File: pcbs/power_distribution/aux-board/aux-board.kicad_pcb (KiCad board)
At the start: 2 copper layers, 85 x 56 mm, 16 parts, among them J1 Conn_01x02, J2 Raspberry Pi - Hat Template -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, J3 Conn_01x03, J4 Conn_01x03, J5 Conn_01x03, J6 Conn_01x03, J7 Conn_01x03, SW1 SW_Push, SW2 SW_Push, U1 YAAJ_WeAct_BlackPill_Part_Like

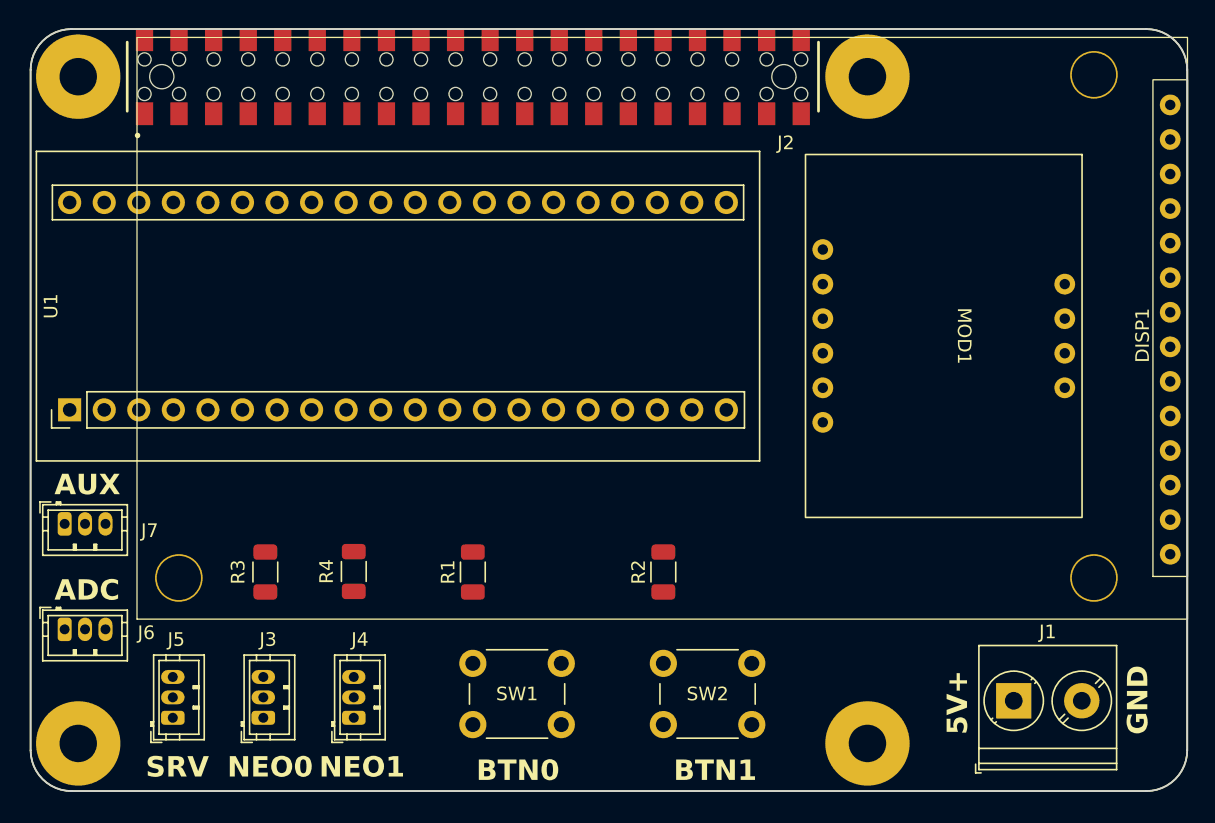
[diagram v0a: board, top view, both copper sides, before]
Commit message: PCB update.
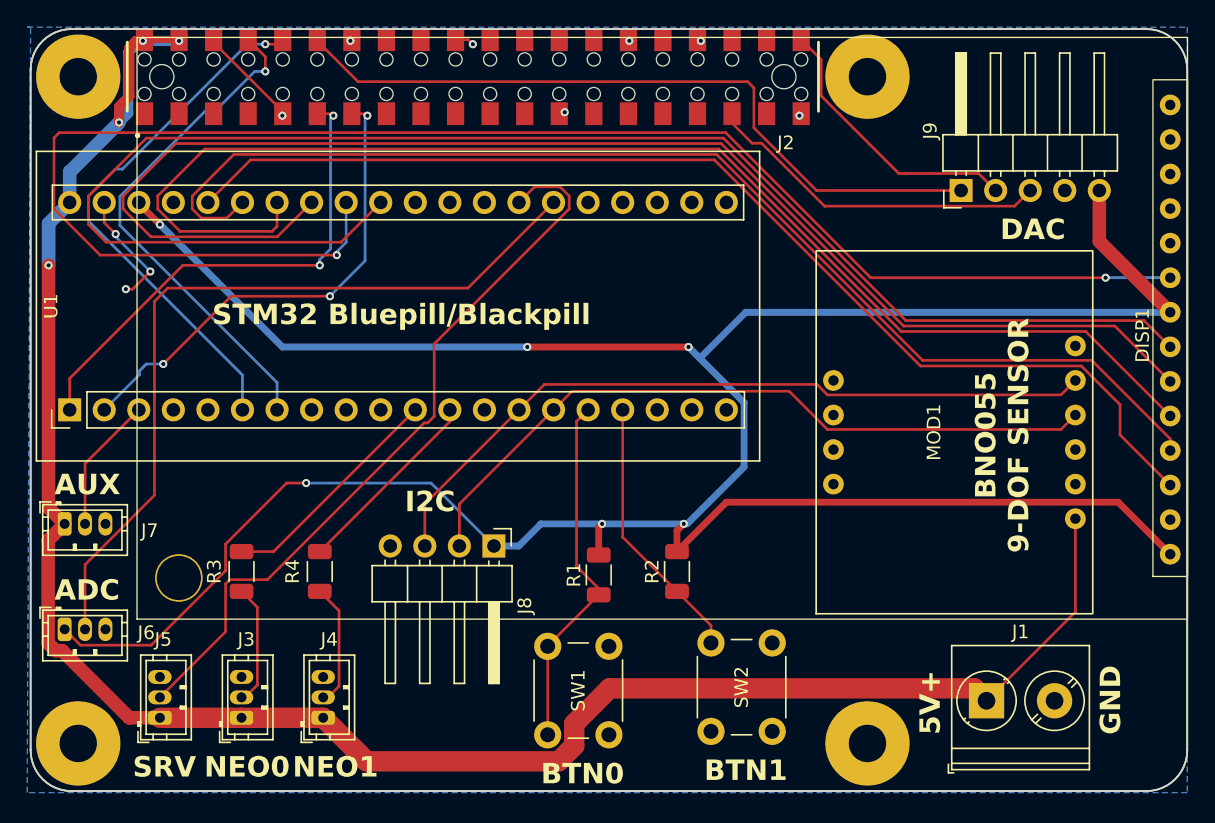
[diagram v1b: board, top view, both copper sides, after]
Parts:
- added J8: Conn_01x04, Connector_PinHeader_2.54mm:PinHeader_1x04_P2.54mm_Horizontal, F.Cu at (71.0, 76.6)
- added J9: Conn_01x05, Connector_PinHeader_2.54mm:PinHeader_1x05_P2.54mm_Horizontal, F.Cu at (105.4, 50.5)
- moved MOD1 27.1 mm to (113.8, 74.6), turned to 90 degrees
- moved R1 9.25 mm to (78.8, 78.8)
- moved SW1 7.60 mm to (75.0, 90.5), turned to 90 degrees
- moved SW2 6.10 mm to (87.0, 90.2), turned to 90 degrees
- moved R4 2.50 mm to (58.2, 78.5)
- moved J4 2.25 mm to (58.5, 89.2)
- moved J1 2.00 mm to (107.2, 88.0)
- moved R3 1.75 mm to (52.5, 78.5)
- moved J3 1.60 mm to (52.5, 89.2)
- moved R2 1.00 mm to (84.5, 78.5)
- moved J5 0.95 mm to (46.5, 89.2)
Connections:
- J2 pad 12: unconnected-(J2-GPIO18-Pad12) -> BCK
- J2 pad 35: unconnected-(J2-GPIO19-Pad35) -> LRCK
- J2 pad 40: unconnected-(J2-GPIO21-Pad40) -> DIN
- J3 pad 3: Net-(J3-Pin_3) -> GND
- J4 pad 3: Net-(J3-Pin_3) -> GND
- J5 pad 3: Net-(J3-Pin_3) -> GND
- J6 pad 2: ADC-1 -> ADC-0
- J7 pad 3: Net-(J3-Pin_3) -> GND
- U1 pad 11: unconnected-(U1-PB3-Pad11) -> NEO-0
- U1 pad 12: unconnected-(U1-PB4-Pad12) -> NEO-1
- U1 pad 16: NEO-0 -> BTN-1
- U1 pad 17: NEO-1 -> BTN-2
- U1 pad 27: unconnected-(U1-PA1-Pad27) -> RC-PWM-0
- U1 pad 5: RC-PWM-0 -> unconnected-(U1-PA8-Pad5)
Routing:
- net +3.3V: track 0.00 -> 207.2 mm, vias 0 -> 6
- net +5V: track 0.00 -> 152.8 mm, vias 0 -> 4
- net TFT-MISO: track 0.00 -> 118.2 mm, vias 0 -> 2
- net TFT-SCK: track 0.00 -> 112.9 mm
- net TFT-MOSI: track 0.00 -> 102.5 mm
- net TFT-DC: track 0.00 -> 96.3 mm
- net TFT-RESET: track 0.00 -> 88.1 mm
- net TFT-CS: track 0.00 -> 83.2 mm
- net ADC-0: track 0.00 -> 58.6 mm
- net RC-PWM-0: track 0.00 -> 55.5 mm
- net SCL: track 0.00 -> 55.3 mm
- net BCK: track 0.00 -> 53.7 mm
- net SDA: track 0.00 -> 53.4 mm
- net Net-(J2-UART0_RX): track 0.00 -> 39.4 mm, vias 0 -> 1
- net Net-(J2-UART0_TX): track 0.00 -> 37.8 mm, vias 0 -> 1
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- added copper zone on B.Cu, net GND
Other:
- board text added: "BNO055 9-DOF SENSOR"
- board text added: "DAC"
- board text added: "ElectroPup Auxiliary Hat metaphasiclabs.com 09/2024"
- board text added: "I2C"
- board text added: "STM32 Bluepill/Blackpill"
